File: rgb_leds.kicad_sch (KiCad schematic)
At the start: 19 parts

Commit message: Use basic parts where possible
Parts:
- C42, C43, C44, C45, C46, C47, C48, C49, C50, C51: footprint Capacitor_SMD:C_0603_1608Metric_Pad1.08x0.95mm_HandSolder -> Capacitor_SMD:C_0603_1608Metric
- R30: footprint Resistor_SMD:R_0603_1608Metric_Pad0.98x0.95mm_HandSolder -> Resistor_SMD:R_0603_1608Metric; LCSC PN C98220 -> C25804
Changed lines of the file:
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@@
 			)
 		)
-		(property "Footprint" "Capacitor_SMD:C_0603_1608Metric_Pad1.08x0.95mm_HandSolder"
+		(property "Footprint" "Capacitor_SMD:C_0603_1608Metric"
 			(at 139.3952 119.38 0)
 			(effects
@@
 			)
 		)
-		(property "Footprint" "Capacitor_SMD:C_0603_1608Metric_Pad1.08x0.95mm_HandSolder"
+		(property "Footprint" "Capacitor_SMD:C_0603_1608Metric"
 			(at 177.4952 119.38 0)
 			(effects
@@
 			)
 		)
-		(property "Footprint" "Resistor_SMD:R_0603_1608Metric_Pad0.98x0.95mm_HandSolder"
+		(property "Footprint" "Resistor_SMD:R_0603_1608Metric"
 			(at 76.962 73.66 90)
 			(effects
@@
 			)
 		)
-		(property "LCSC PN" "C98220"
+		(property "LCSC PN" "C25804"
 			(at 78.74 73.66 0)
 			(effects
@@
 			)
 		)
-		(property "Footprint" "Capacitor_SMD:C_0603_1608Metric_Pad1.08x0.95mm_HandSolder"
+		(property "Footprint" "Capacitor_SMD:C_0603_1608Metric"
 			(at 113.9952 119.38 0)
 			(effects
@@
 			)
 		)
-		(property "Footprint" "Capacitor_SMD:C_0603_1608Metric_Pad1.08x0.95mm_HandSolder"
+		(property "Footprint" "Capacitor_SMD:C_0603_1608Metric"
 			(at 88.5952 119.38 0)
 			(effects
@@
 			)
 		)
-		(property "Footprint" "Capacitor_SMD:C_0603_1608Metric_Pad1.08x0.95mm_HandSolder"
+		(property "Footprint" "Capacitor_SMD:C_0603_1608Metric"
 			(at 190.1952 119.38 0)
 			(effects
@@
 			)
 		)
-		(property "Footprint" "Capacitor_SMD:C_0603_1608Metric_Pad1.08x0.95mm_HandSolder"
+		(property "Footprint" "Capacitor_SMD:C_0603_1608Metric"
 			(at 126.6952 119.38 0)
 			(effects
@@
 			)
 		)
-		(property "Footprint" "Capacitor_SMD:C_0603_1608Metric_Pad1.08x0.95mm_HandSolder"
+		(property "Footprint" "Capacitor_SMD:C_0603_1608Metric"
 			(at 164.7952 119.38 0)
 			(effects
@@
 			)
 		)
-		(property "Footprint" "Capacitor_SMD:C_0603_1608Metric_Pad1.08x0.95mm_HandSolder"
+		(property "Footprint" "Capacitor_SMD:C_0603_1608Metric"
 			(at 152.0952 119.38 0)
 			(effects
@@
 			)
 		)
-		(property "Footprint" "Capacitor_SMD:C_0603_1608Metric_Pad1.08x0.95mm_HandSolder"
+		(property "Footprint" "Capacitor_SMD:C_0603_1608Metric"
 			(at 202.8952 119.38 0)
 			(effects
@@
 			)
 		)
-		(property "Footprint" "Capacitor_SMD:C_0603_1608Metric_Pad1.08x0.95mm_HandSolder"
+		(property "Footprint" "Capacitor_SMD:C_0603_1608Metric"
 			(at 101.2952 119.38 0)
 			(effects

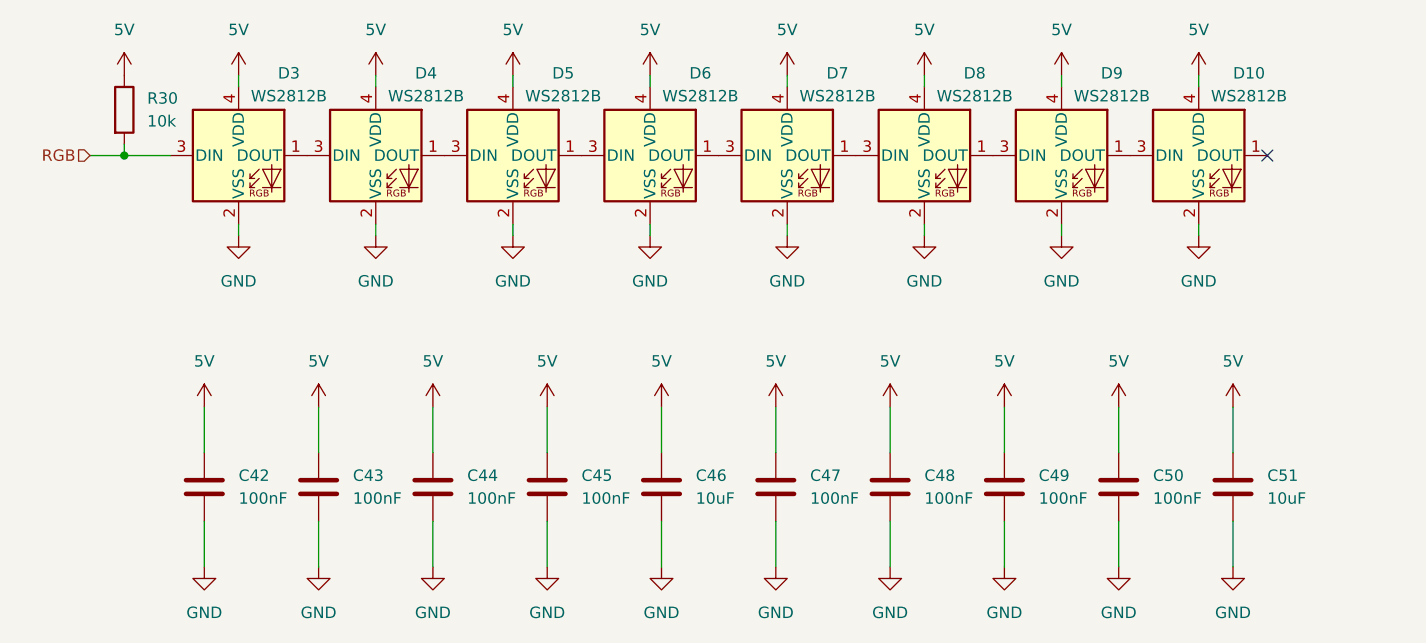
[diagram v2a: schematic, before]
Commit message: Sketch out component placement
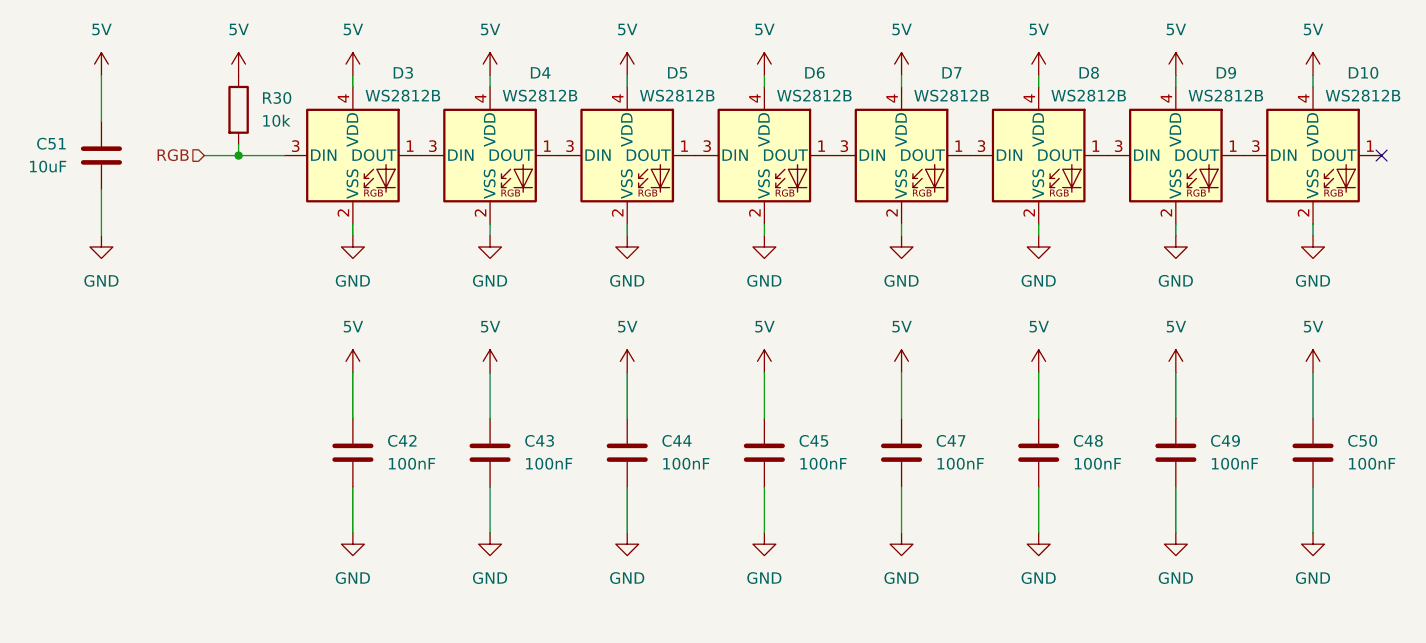
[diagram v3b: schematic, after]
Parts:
- removed C46: 10uF, Capacitor_SMD:C_0603_1608Metric, symbol Device:C
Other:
- moved on the sheet: C42, C43, C44, C45, C47, C48, C49, C50, C51, D10, D3, D4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
